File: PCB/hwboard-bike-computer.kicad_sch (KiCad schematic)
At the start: 0 parts

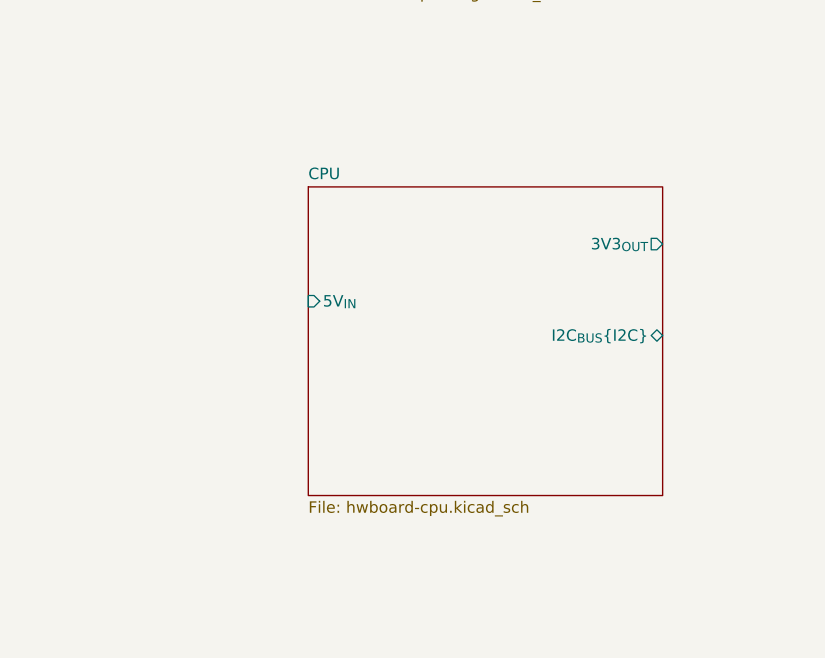
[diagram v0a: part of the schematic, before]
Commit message: add sensors
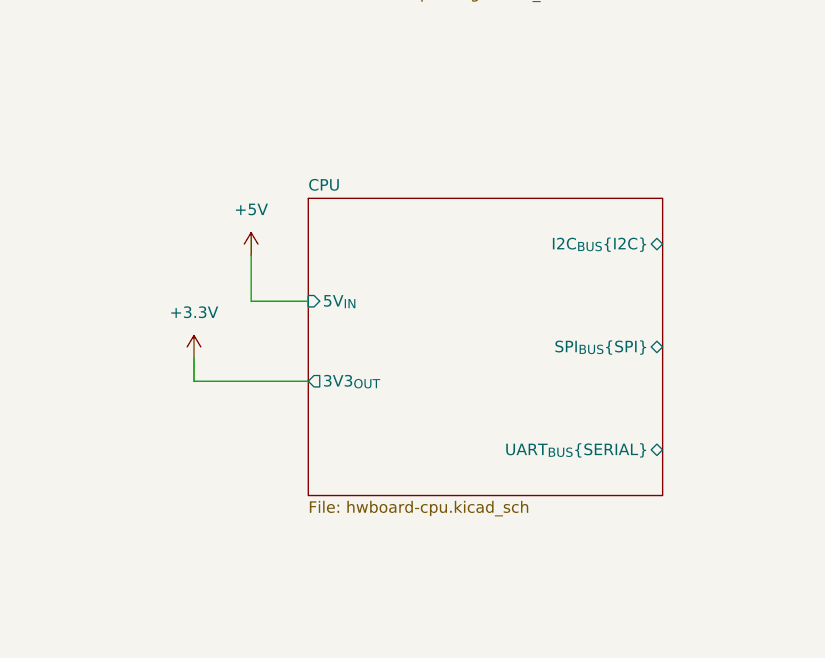
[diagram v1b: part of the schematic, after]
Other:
- sheet CPU ports: added SPI_{BUS}{SPI}, UART_{BUS}{SERIAL}; removed none
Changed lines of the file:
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@@
+	(wire
+		(pts
+			(xy 116.84 104.14) (xy 116.84 106.68)
+		)
+		(stroke
+			(width 0)
+			(type default)
+		)
+	)
 	(wire
 		(pts
@@
 		(pts
 			(xy 250.19 38.1) (xy 245.11 38.1)
+		)
+		(stroke
+			(width 0)
+			(type default)
+		)
+	)
+	(wire
+		(pts
+			(xy 123.19 92.71) (xy 123.19 97.79)
+		)
+		(stroke
+			(width 0)
+			(type default)
+		)
+	)
+	(wire
+		(pts
+			(xy 116.84 106.68) (xy 129.54 106.68)
+		)
+		(stroke
+			(width 0)
+			(type default)
+		)
+	)
+	(wire
+		(pts
+			(xy 123.19 97.79) (xy 129.54 97.79)
 		)
 		(stroke
@@
 		)
 	)
+	(symbol
+		(lib_id "power:+3.3V")
+		(at 116.84 104.14 0)
+		(unit 1)
+		(exclude_from_sim no)
+		(in_bom yes)
+		(on_board yes)
+		(dnp no)
+		(fields_autoplaced yes)
+		(property "Reference" "#PWR02"
+			(at 116.84 107.95 0)
+			(effects
+				(font
+					(size 1.27 1.27)
+				)
+				(hide yes)
+			)
+		)
+		(property "Value" "+3.3V"
+			(at 116.84 99.06 0)
+			(effects
+				(font
+					(size 1.27 1.27)
+				)
+			)
+		)
+		(property "Footprint" ""
+			(at 116.84 104.14 0)
+			(effects
+				(font
+					(size 1.27 1.27)
+				)
+				(hide yes)
+			)
+		)
+		(property "Datasheet" ""
+			(at 116.84 104.14 0)
+			(effects
+				(font
+					(size 1.27 1.27)
+				)
+				(hide yes)
+			)
+		)
+		(property "Description" "Power symbol creates a global label with name \"+3.3V\""
+			(at 116.84 104.14 0)
+			(effects
+				(font
+					(size 1.27 1.27)
+				)
+				(hide yes)
+			)
+		)
+		(pin "1"
+		)
+		(instances
+			(project ""
+				(path "/8c0f76b9-ee42-4bcf-bb95-09772e367402"
+					(reference "#PWR02")
+					(unit 1)
+				)
+			)
+		)
+	)
+	(symbol
+		(lib_id "power:+5V")
+		(at 123.19 92.71 0)
+		(unit 1)
+		(exclude_from_sim no)
+		(in_bom yes)
+		(on_board yes)
+		(dnp no)
+		(fields_autoplaced yes)
+		(property "Reference" "#PWR01"
+			(at 123.19 96.52 0)
+			(effects
+				(font
+					(size 1.27 1.27)
+				)
+				(hide yes)
+			)
+		)
+		(property "Value" "+5V"
+			(at 123.19 87.63 0)
+			(effects
+				(font
+					(size 1.27 1.27)
+				)
+			)
+		)
+		(property "Footprint" ""
+			(at 123.19 92.71 0)
+			(effects
+				(font
+					(size 1.27 1.27)
+				)
+				(hide yes)
+			)
+		)
+		(property "Datasheet" ""
+			(at 123.19 92.71 0)
+			(effects
+				(font
+					(size 1.27 1.27)
+				)
+				(hide yes)
+			)
+		)
+		(property "Description" "Power symbol creates a global label with name \"+5V\""
+			(at 123.19 92.71 0)
+			(effects
+				(font
+					(size 1.27 1.27)
+				)
+				(hide yes)
+			)
+		)
+		(pin "1"
+		)
+		(instances
+			(project "hwboard-bike-computer"
+				(path "/8c0f76b9-ee42-4bcf-bb95-09772e367402"
+					(reference "#PWR01")
+					(unit 1)
+				)
+			)
+		)
+	)
 	(sheet
 		(at 52.07 142.24)
@@
 	)
 	(sheet
-		(at 129.54 85.09)
-		(size 39.37 34.29)
+		(at 129.54 86.36)
+		(size 39.37 33.02)
 		(exclude_from_sim no)
 		(in_bom yes)
@@
 		)
 		(property "Sheetname" "CPU"
-			(at 129.54 84.3784 0)
+			(at 129.54 85.6484 0)
 			(effects
 				(font
@@
 		)
 		(pin "3V3_{OUT}" output
+			(at 129.54 106.68 180)
+			(effects
+				(font
+					(size 1.27 1.27)
+				)
+				(justify left)
+			)
+		)
+		(pin "I2C_{BUS}{I2C}" bidirectional
 			(at 168.91 91.44 0)
-			(effects
-				(font
-					(size 1.27 1.27)
-				)
-				(justify right)
-			)
-		)
-		(pin "I2C_{BUS}{I2C}" bidirectional
-			(at 168.91 101.6 0)
 			(effects
 				(font
@@
 			)
 		)
+		(pin "SPI_{BUS}{SPI}" bidirectional
+			(at 168.91 102.87 0)
+			(effects
+				(font
+					(size 1.27 1.27)
+				)
+				(justify right)
+			)
+		)
+		(pin "UART_{BUS}{SERIAL}" bidirectional
+			(at 168.91 114.3 0)
+			(effects
+				(font
+					(size 1.27 1.27)
+				)
+				(justify right)
+			)
+		)
